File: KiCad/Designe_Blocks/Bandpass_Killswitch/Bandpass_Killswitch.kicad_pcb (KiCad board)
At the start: 4 copper layers, 53 parts, among them J1 Stecker_In_Out_Switch, J2 Conn_02x07_Odd_Even, U1 TL074, U2 TL074

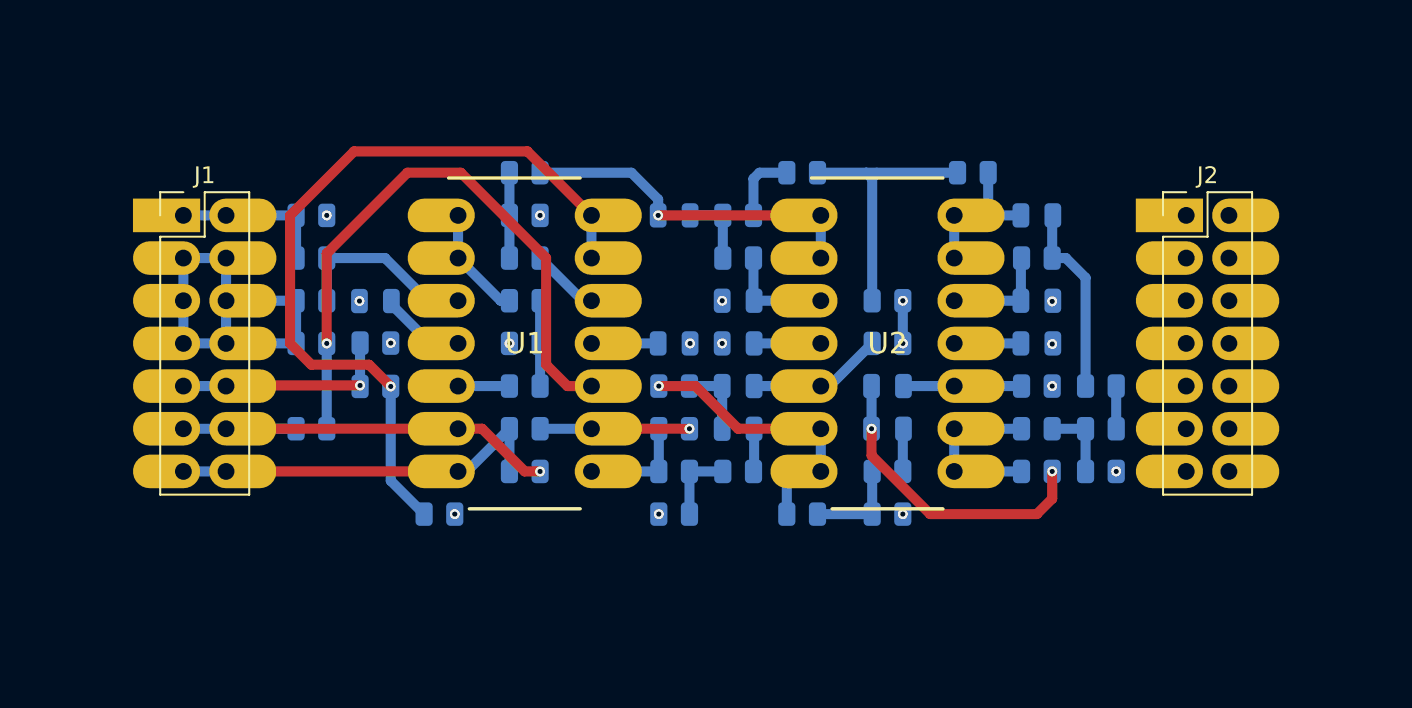
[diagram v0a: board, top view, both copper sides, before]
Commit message: Update
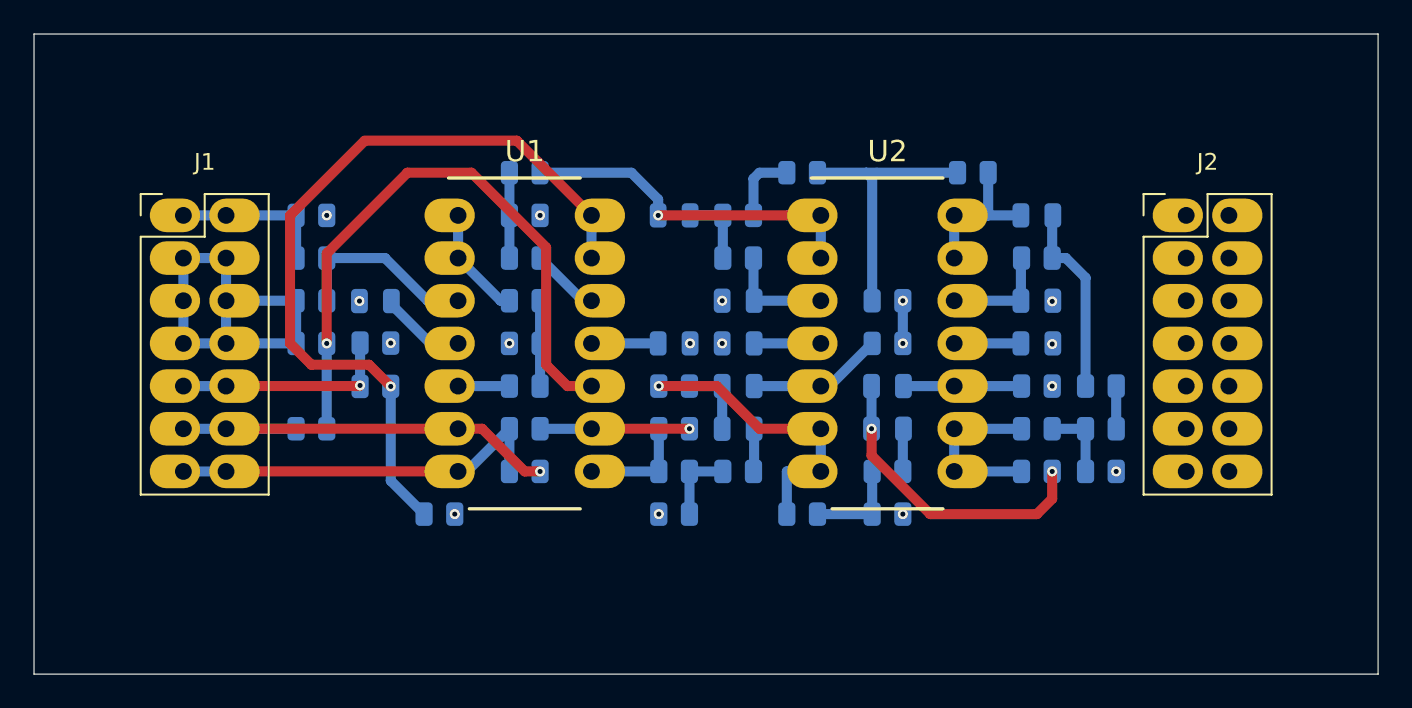
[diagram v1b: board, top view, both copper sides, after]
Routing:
- net Net-(U1D--): track 46.7 -> 47.3 mm
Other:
- board outline added: 80 x 38.1 mm
